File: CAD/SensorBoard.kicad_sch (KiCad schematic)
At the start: 18 parts, among them SW1 BOOT_SW, X1 32MHz, X2 32kHz768

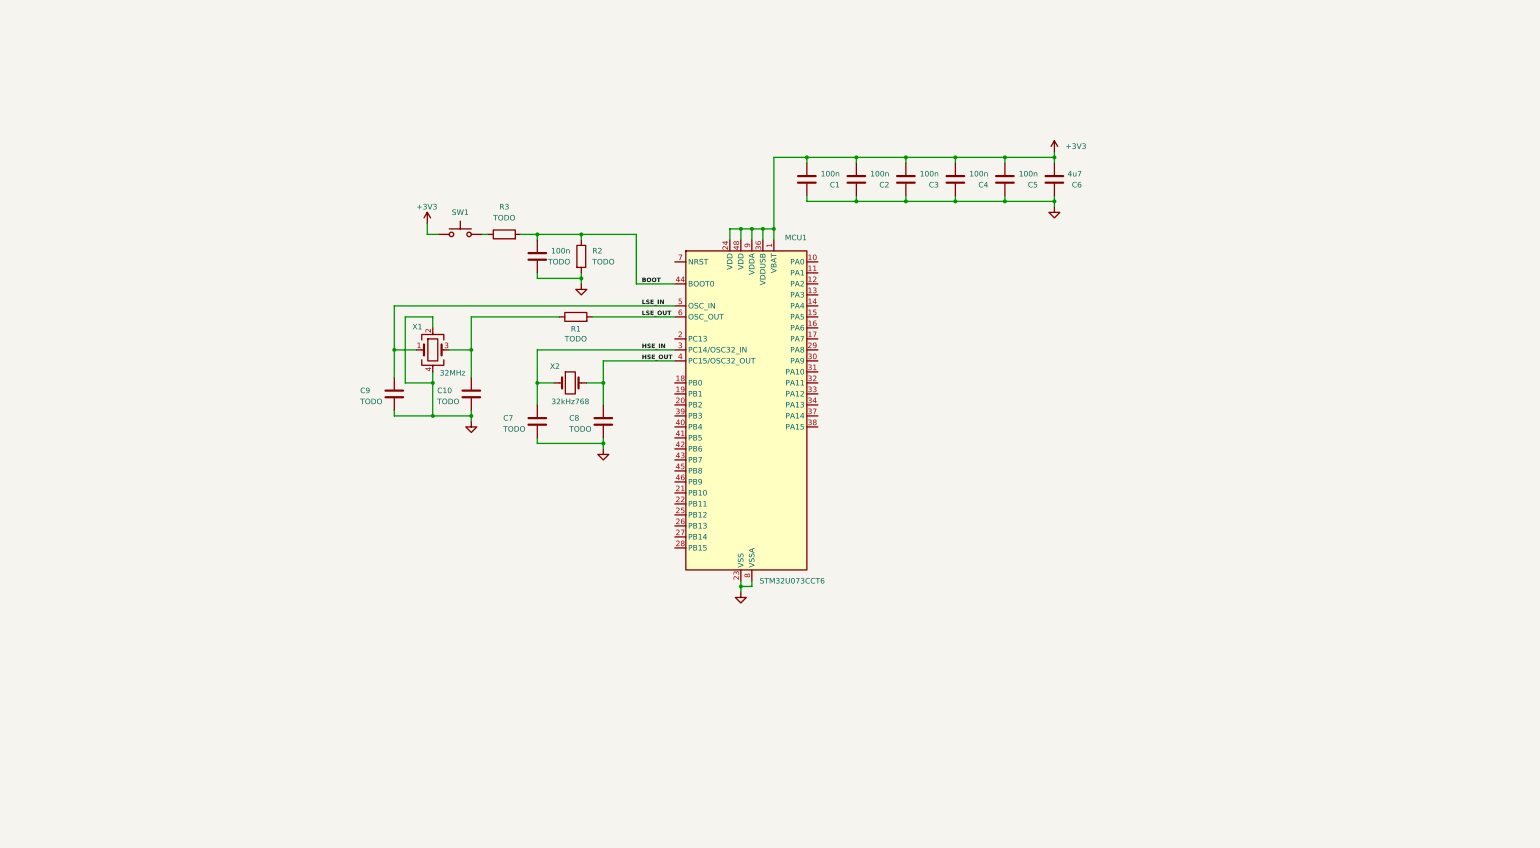
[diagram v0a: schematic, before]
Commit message: Further progress with power and peripherals
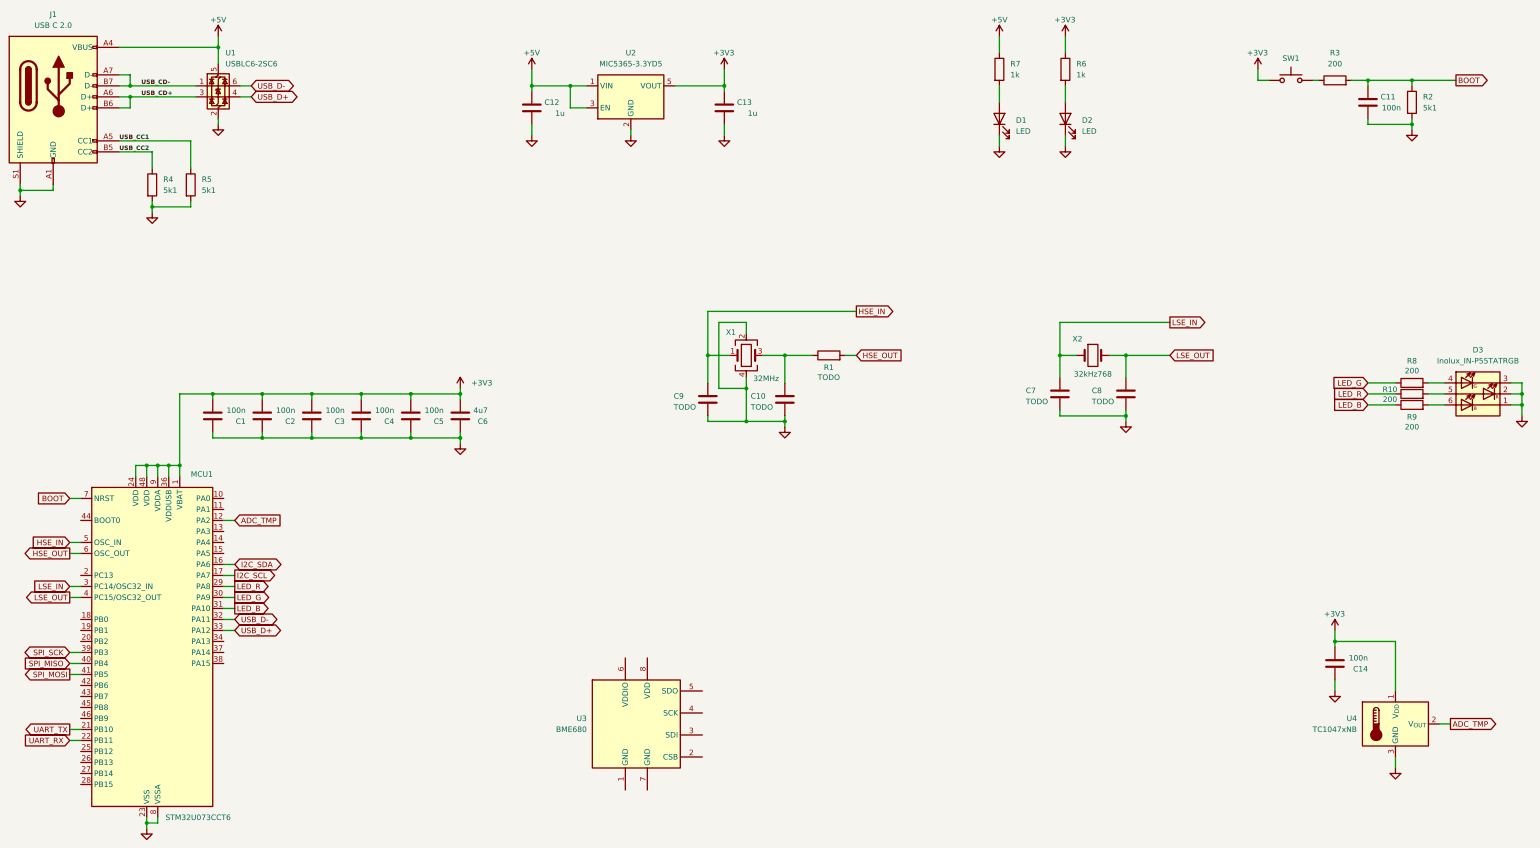
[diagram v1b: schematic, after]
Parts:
- added C12, C13: 1u, symbol Device:C
- added C14: 100n, symbol Device:C
- added D1, D2: LED, symbol Device:LED
- added D3: Inolux_IN-P55TATRGB, LED_SMD:LED_Inolux_IN-P55TATRGB_PLCC6_5.0x5.5mm_P1.8mm, symbol LED:Inolux_IN-P55TATRGB
- added J1: USB C 2.0, symbol SensorBoard:USB_C_Receptacle_USB2.0
- added R10, R8, R9: 200, symbol Device:R
- added R4, R5: 5k1, symbol Device:R
- added R6, R7: 1k, symbol Device:R
- added U1: USBLC6-2SC6, Package_TO_SOT_SMD:SOT-23-6, symbol Power_Protection:USBLC6-2SC6
- added U2: MIC5365-3.3YD5, Package_TO_SOT_SMD:SOT-23-5, symbol Regulator_Linear:MIC5365-3.3YD5
- added U3: BME680, Package_LGA:Bosch_LGA-8_3x3mm_P0.8mm_ClockwisePinNumbering, symbol Sensor:BME680
- added U4: TC1047xNB, Package_TO_SOT_SMD:SOT-23, symbol Sensor_Temperature:TC1047xNB
- R2: value TODO -> 5k1
- R3: value TODO -> 200
- renumbered TODO to C11
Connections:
- net +3V3: now also C13.2, C14.2, R6.1, U2.5 (VOUT), U4.1 (V_{DD})
- net BOOT: now also MCU1.7 (NRST); no longer MCU1.44 (BOOT0)
- net GND: now also C12.1, C13.1, C14.1, D1.1 (K), D2.1 (K), D3.1 (KB), D3.2 (KR), D3.3 (KG), J1.A1 (GND), J1.A12 (GND), J1.B1 (GND), J1.B12 (GND), J1.S1 (SHIELD), R4.2, R5.2, U1.2 (GND), U2.2 (GND), U4.3 (GND)
- net HSE_IN: now also C9.1, MCU1.5 (OSC_IN), X1.1; no longer C7.1, MCU1.3 (PC14/OSC32_IN), X2.1
- net HSE_OUT: now also MCU1.6 (OSC_OUT), R1.2; no longer C8.1, MCU1.4 (PC15/OSC32_OUT), X2.2
- net LSE_IN: now also C7.1, MCU1.3 (PC14/OSC32_IN), X2.1; no longer C9.1, MCU1.5 (OSC_IN), X1.1
- net LSE_OUT: now also C8.1, MCU1.4 (PC15/OSC32_OUT), X2.2; no longer MCU1.6 (OSC_OUT), R1.2
- net ADC_TMP: now reaches MCU1.12 (PA2)
- net ADC_TMP: now also U4.2 (V_{OUT})
- net I2C_SDA: now reaches MCU1.16 (PA6)
- net I2C_SCL: now reaches MCU1.17 (PA7)
- net UART_TX: now reaches MCU1.21 (PB10)
- net UART_RX: now reaches MCU1.22 (PB11)
- net LED_R: now reaches MCU1.29 (PA8)
- net LED_R: now also R10.1
- net LED_G: now reaches MCU1.30 (PA9)
- net LED_G: now also R8.1
- net LED_B: now reaches MCU1.31 (PA10)
- net LED_B: now also R9.1
- net USB_D-: now reaches MCU1.32 (PA11)
- net USB_D-: now also U1.6 (I/O1)
- net USB_D+: now reaches MCU1.33 (PA12)
- net USB_D+: now also U1.4 (I/O2)
- net SPI_SCK: now reaches MCU1.39 (PB3)
- net SPI_MISO: now reaches MCU1.40 (PB4)
- net SPI_MOSI: now reaches MCU1.41 (PB5)
- new net: D3.5 (AR), R10.2
- new net: D3.4 (AG), R8.2
- new net: D2.2 (A), R6.2
- new net: D3.6 (AB), R9.2
- new net: D1.2 (A), R7.2
- new net +5V: C12.2, J1.A4 (VBUS), J1.A9 (VBUS), J1.B4 (VBUS), J1.B9 (VBUS), R7.1, U1.5 (VBUS), U2.1 (VIN), U2.3 (EN)
- new net USB_CC1: J1.A5 (CC1), R5.1
- new net USB_CC2: J1.B5 (CC2), R4.1
- new net USB_CD+: J1.A6 (D+), J1.B6 (D+), U1.3 (I/O2)
- new net USB_CD-: J1.A7 (D-), J1.B7 (D-), U1.1 (I/O1)
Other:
- moved on the sheet: C1, C10, C11, C2, C3, C4, C5, C6, C7, C8, C9, MCU1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
